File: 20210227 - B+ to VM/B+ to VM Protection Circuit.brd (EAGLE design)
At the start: 46 parts, among them Q1 SOT23, Q4 SOT23, Q5 DPACK

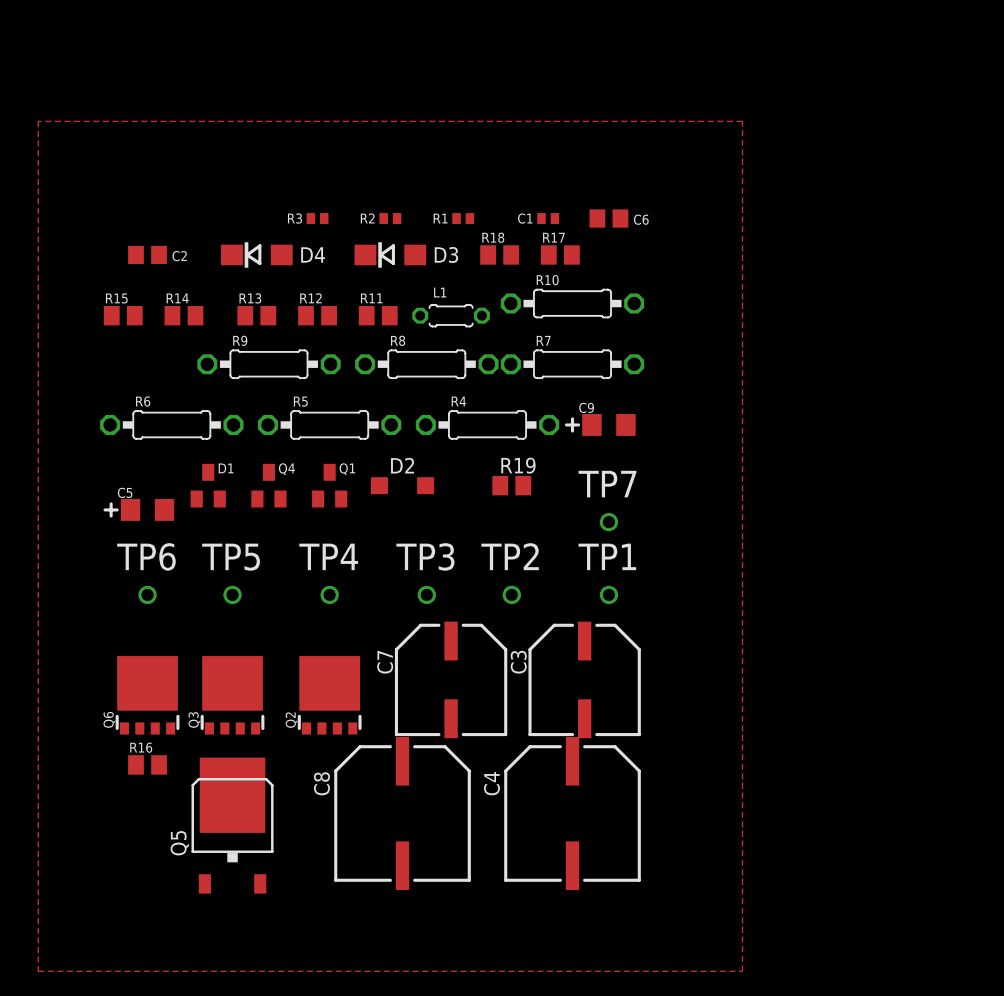
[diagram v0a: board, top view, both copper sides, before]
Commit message: 02MAR2021
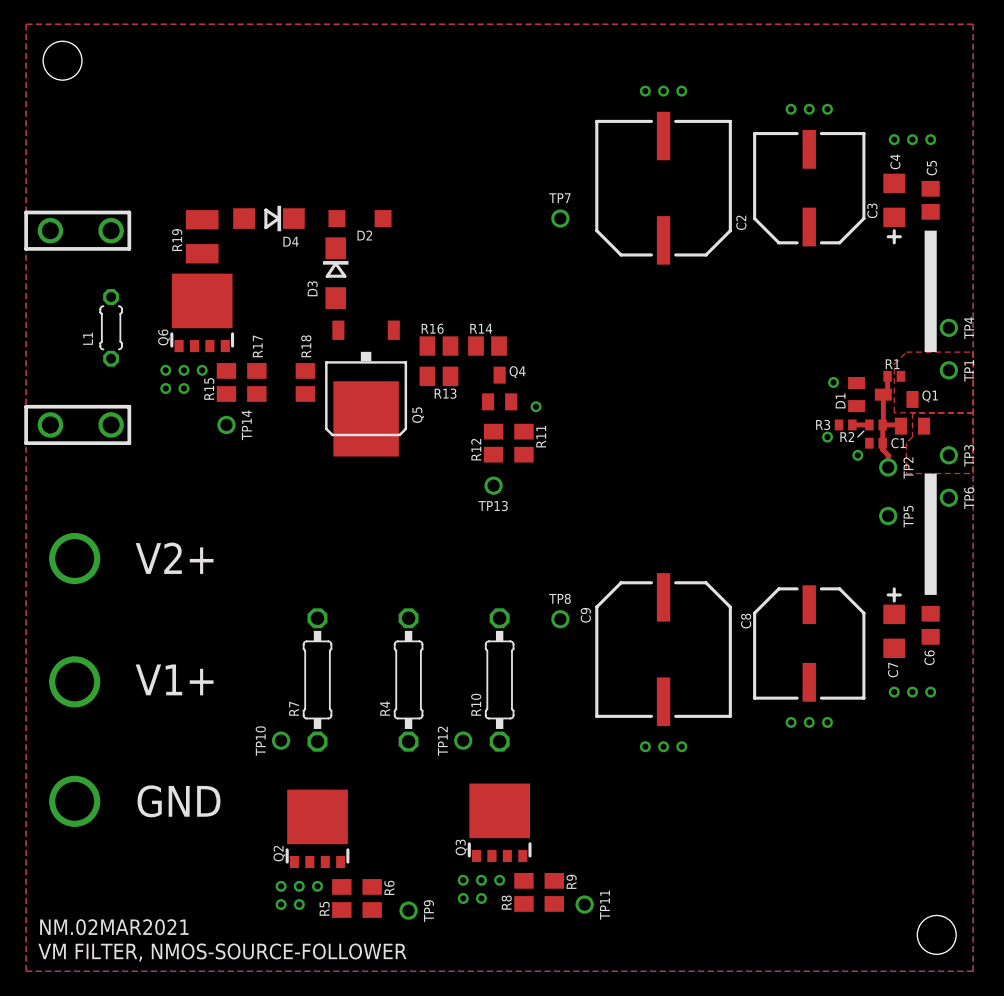
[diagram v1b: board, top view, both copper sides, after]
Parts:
- added NM.02MAR2021: VM FILTER, NMOS-SOURCE-FOLLOWER, nolan:EVAL-80X80
- added TP10, TP11, TP12, TP13, TP14, TP8, TP9: TESTPOINTKE5000-SMTEXT, nolan:PINS_1_TESTPOINT_KE5000_NOTEXT
- added U$1, U$2: SPADE-TAB, nolan:SPADE-TAB-6.3MM
- C2: value 0805 -> PCR-10X8; device nolan:C0805 -> nolan:C-PCR-10X8
- C4: value PCR-10X8 -> 1206; device nolan:C-PCR-10X8 -> nolan:C1206
- C5: value 1206 -> 0805; device nolan:C1206 -> nolan:C0805
- C7: value PCR-8X7 -> 1206; device nolan:C-PCR-8X7 -> nolan:C1206
- C8: value PCR-10X8 -> PCR-8X7; device nolan:C-PCR-10X8 -> nolan:C-PCR-8X7
- C9: value 1206 -> PCR-10X8; device nolan:C1206 -> nolan:C-PCR-10X8
- R19: device nolan:M2012 -> nolan:R1210
- R5, R6, R8, R9: device nolan:0207/10 -> nolan:M0805
- TP1, TP2, TP3, TP4, TP5, TP6, TP7: value TESTPOINTKE5000 -> TESTPOINTKE5000-SMTEXT; device nolan:PINS_1_TESTPOINT_KE5000 -> nolan:PINS_1_TESTPOINT_KE5000_NOTEXT
- moved C5 69.4 mm to (75.5, 64.5), turned to 90 degrees
- moved TP6 66.5 mm to (77.0, 40.0), turned to 270 degrees
- moved C4 57.0 mm to (72.5, 64.5), turned to 90 degrees
- moved TP4 55.5 mm to (77.0, 54.0), turned to 270 degrees
- moved D1 55.0 mm to (70.5, 48.5), turned to 270 degrees
- moved TP5 54.4 mm to (72.0, 38.5), turned to 270 degrees
- moved R9 49.4 mm to (44.5, 7.50), turned to 270 degrees
- moved Q1 48.4 mm to (74.0, 47.0)
- moved R3 46.7 mm to (68.5, 46.0)
- moved C3 44.5 mm to (65.5, 65.5), turned to 180 degrees
- moved TP3 44.5 mm to (77.0, 43.5), turned to 270 degrees
- moved R8 44.2 mm to (42.0, 7.50), turned to 270 degrees
- moved R2 43.5 mm to (71.0, 46.0)
- moved C2 42.9 mm to (53.5, 65.5), turned to 180 degrees
- moved C6 42.7 mm to (75.5, 29.5), turned to 270 degrees
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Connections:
- net B+: now also TP7.1; no longer TP4.1
- net GND: now also C2.-, C5.2, NM.02MAR2021.GND, R11.2, R18.2, R5.1, TP4.1, TP5.1, TP6.1; no longer C2.2, C5.-, R14.2, R17.2, R7.1
- net HIGH_VOLTAGE: now also NM.02MAR2021.V1+, R13.1; no longer R12.1
- net HIGH_VOLTAGE_CONTROL_1: now also R11.1, R12.1, TP13.1; no longer R13.1, R14.1
- net LOAD_CONTROL_1: now also R5.2, R6.2, TP9.1; no longer R10.2, R7.2
- net LOAD_CONTROL_2: now also TP11.1
- net N$10: now also D3.A, R18.1; no longer D4.A, R15.1
- net N$11: now also R17.2; no longer R16.2
- net N$12: now also D4.A, U$2.P$1, U$2.P$2; no longer D3.A
- net N$13: now also R16.1; no longer R11.1
- net N$2: now also R7.1, TP10.1; no longer R5.1, TP5.1
- net N$3: now also R10.1, TP12.1; no longer R6.1, TP6.1
- net N$6: now also R6.1; no longer R10.1
- net N$7: now also R13.2, R14.1, R16.2; no longer R11.2, R12.2, R18.1
- net N$8: now also R12.2; no longer R13.2
- net N$9: now also R14.2; no longer R18.2
- net Q1.DRAIN: now also C2.+, C5.1; no longer C2.1, C5.+
- net SPIKE_VOLTAGE_CONTROL_2: now also R15.1, TP14.1; no longer R16.1
- net VIN: now also NM.02MAR2021.V2+, U$1.P$1, U$1.P$2
- net VM: now also R10.2, R7.2, TP8.1; no longer R5.2, R6.2, TP7.1
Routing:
- net Q1.GATE: track 0.00 -> 9.39 mm
- net N$4: track 0.00 -> 1.40 mm
- added copper zone on layer 16, net GND
- added copper zone on layer 1, net Q1.DRAIN
- added copper zone on layer 1, net VM
